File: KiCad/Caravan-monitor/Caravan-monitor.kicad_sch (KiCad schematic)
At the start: 14 parts, among them IC2 STM32L011F4P6TR, J1 Conn_ARM_JTAG_SWD_20, J2 8-28V input, SW1 SW_SPST

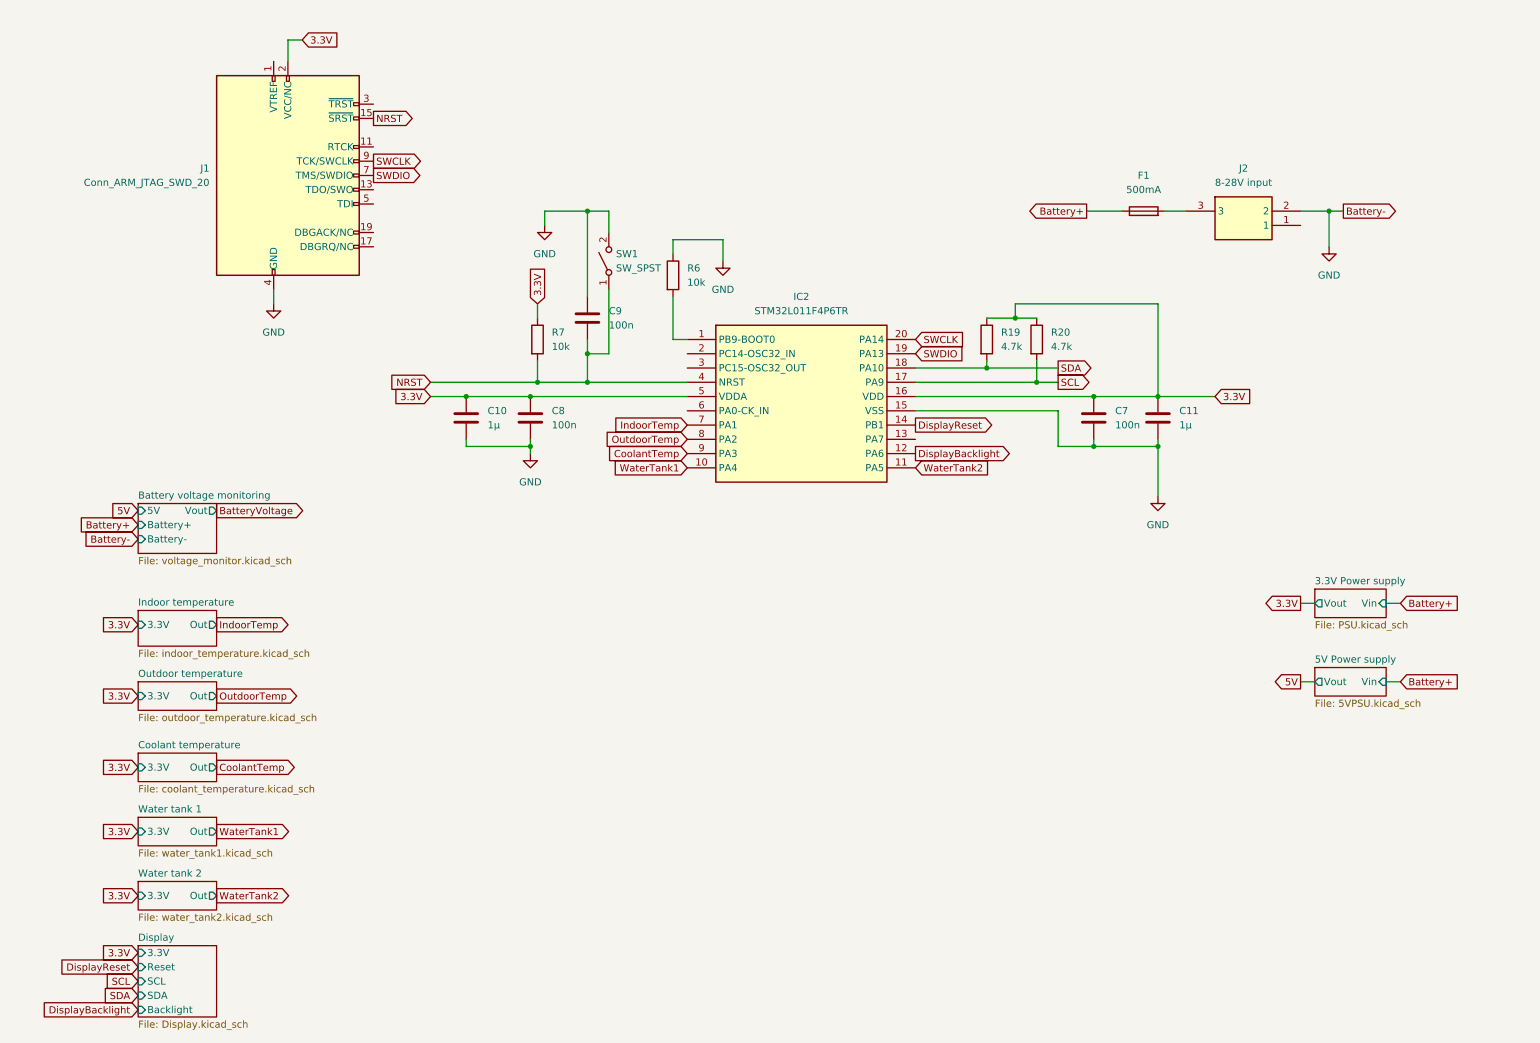
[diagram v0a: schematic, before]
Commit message: Schematics done
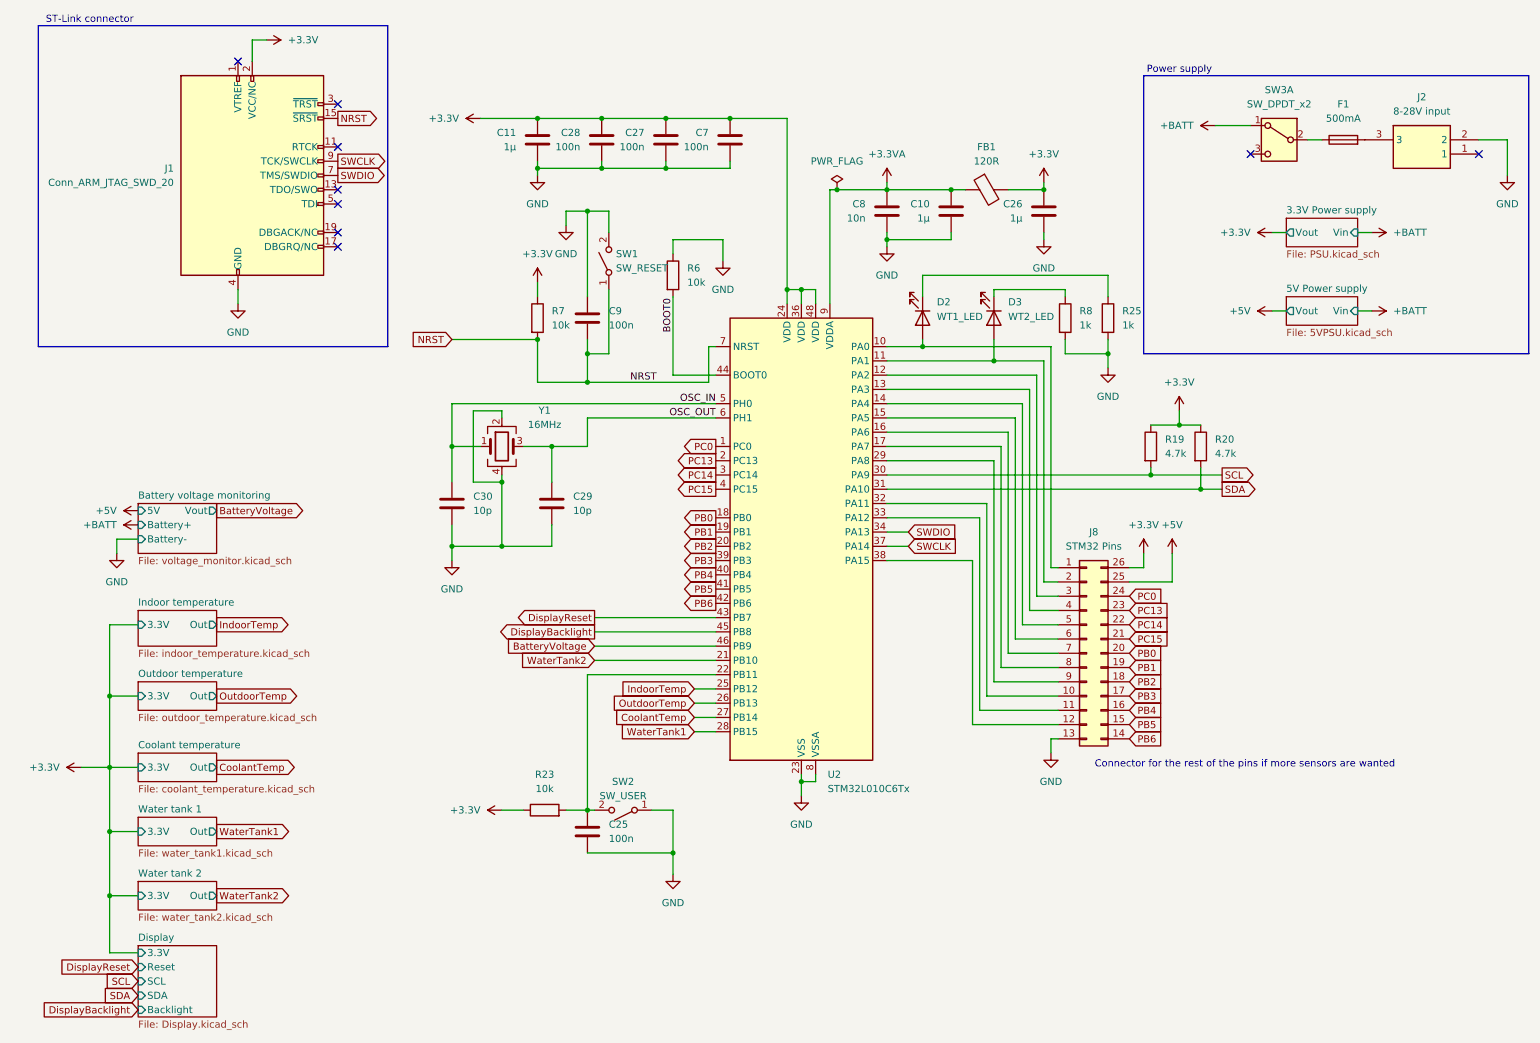
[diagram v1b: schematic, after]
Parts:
- removed IC2: STM32L011F4P6TR, SamacSys_Parts:SOP65P640X120-20N, symbol SamacSys_Parts:STM32L011F4P6TR
- added C25, C27, C28: 100n, Capacitor_SMD:C_0402_1005Metric_Pad0.74x0.62mm_HandSolder, symbol Device:C
- added C26: 1µ, Capacitor_SMD:C_0402_1005Metric_Pad0.74x0.62mm_HandSolder, symbol Device:C
- added C29, C30: 10p, Capacitor_SMD:C_0402_1005Metric_Pad0.74x0.62mm_HandSolder, symbol Device:C
- added D2: WT1_LED, LED_SMD:LED_0402_1005Metric_Pad0.77x0.64mm_HandSolder, symbol Device:LED
- added D3: WT2_LED, LED_SMD:LED_0402_1005Metric_Pad0.77x0.64mm_HandSolder, symbol Device:LED
- added FB1: 120R, Inductor_SMD:L_0402_1005Metric_Pad0.77x0.64mm_HandSolder, symbol Device:FerriteBead
- added J8: STM32 Pins, Connector_PinHeader_2.54mm:PinHeader_2x13_P2.54mm_Horizontal, symbol Connector_Generic:Conn_02x13_Counter_Clockwise
- added R23: 10k, Resistor_SMD:R_0402_1005Metric_Pad0.72x0.64mm_HandSolder, symbol Device:R
- added R25, R8: 1k, Resistor_SMD:R_0402_1005Metric_Pad0.72x0.64mm_HandSolder, symbol Device:R
- added SW2: SW_USER, Button_Switch_SMD:SW_SPST_PTS645, symbol Switch:SW_SPST
- added SW3: SW_DPDT_x2, Button_Switch_THT:SW_E-Switch_EG2219_DPDT_Angled, symbol Switch:SW_DPDT_x2
- added U2: STM32L010C6Tx, Package_QFP:LQFP-48_7x7mm_P0.5mm, symbol MCU_ST_STM32L0:STM32L010C6Tx
- added Y1: 16MHz, symbol Device:Crystal_GND24
- C10, C11, C7, C9: footprint Capacitor_SMD:C_0805_2012Metric_Pad1.18x1.45mm_HandSolder -> Capacitor_SMD:C_0402_1005Metric_Pad0.74x0.62mm_HandSolder
- C8: value 100n -> 10n; footprint Capacitor_SMD:C_0805_2012Metric_Pad1.18x1.45mm_HandSolder -> Capacitor_SMD:C_0402_1005Metric_Pad0.74x0.62mm_HandSolder
- R19, R20, R6, R7: footprint Resistor_SMD:R_0805_2012Metric_Pad1.20x1.40mm_HandSolder -> Resistor_SMD:R_0402_1005Metric_Pad0.72x0.64mm_HandSolder
- SW1: value SW_SPST -> SW_RESET
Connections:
- net BatteryVoltage: now also U2.46 (PB9)
- net CoolantTemp: now also U2.27 (PB14)
- net DisplayBacklight: now also U2.45 (PB8)
- net DisplayReset: now also U2.43 (PB7)
- net GND: now also C25.1, C26.2, C27.2, C28.2, C29.2, C30.2, J8.13 (Pin_13), R25.2, R8.2, SW2.1 (A), U2.23 (VSS), U2.35 (VSS), U2.47 (VSS), U2.8 (VSSA), Y1.2, Y1.4
- net IndoorTemp: now also U2.25 (PB12)
- net NRST: now also U2.7 (NRST)
- net OutdoorTemp: now also U2.26 (PB13)
- net SCL: now also R19.2, U2.30 (PA9); no longer R20.2
- net SDA: now also R20.2, U2.31 (PA10); no longer R19.2
- net SWCLK: now also U2.37 (PA14)
- net SWDIO: now also U2.34 (PA13)
- net WaterTank1: now also U2.28 (PB15)
- net WaterTank2: now also U2.21 (PB10)
- net BOOT0: now reaches R6.2
- net BOOT0: now also U2.44 (BOOT0)
- net 3.3V renamed +3.3V
- net +3.3V: now also C26.1, C27.1, C28.1, FB1.2, J8.26 (Pin_26), R23.1, U2.24 (VDD), U2.36 (VDD), U2.48 (VDD); no longer C10.1, C8.1
- net Battery+: no longer names the net of F1.1
- net Battery+: now also SW3.2 (B)
- new net: D2.2 (A), J8.1 (Pin_1), U2.10 (PA0)
- new net: J8.10 (Pin_10), U2.32 (PA11)
- new net: J8.11 (Pin_11), U2.33 (PA12)
- new net: J8.12 (Pin_12), U2.38 (PA15)
- new net: D3.2 (A), J8.2 (Pin_2), U2.11 (PA1)
- new net: J8.3 (Pin_3), U2.12 (PA2)
- new net: J8.4 (Pin_4), U2.13 (PA3)
- new net: J8.5 (Pin_5), U2.14 (PA4)
- new net: J8.6 (Pin_6), U2.15 (PA5)
- new net: J8.7 (Pin_7), U2.16 (PA6)
- new net: J8.8 (Pin_8), U2.17 (PA7)
- new net: J8.9 (Pin_9), U2.29 (PA8)
- new net: C25.2, R23.2, SW2.2 (B), U2.22 (PB11)
- new net: D3.1 (K), R8.1
- new net: D2.1 (K), R25.1
- new net +3.3VA: C10.1, C8.1, FB1.1, U2.9 (VDDA)
- new net +5V: J8.25 (Pin_25)
- new net +BATT: SW3.1 (A)
- new net OSC_IN: C30.1, U2.5 (PH0), Y1.1
- new net OSC_OUT: C29.1, U2.6 (PH1), Y1.3
- new net PB0: J8.20 (Pin_20), U2.18 (PB0)
- new net PB1: J8.19 (Pin_19), U2.19 (PB1)
- new net PB2: J8.18 (Pin_18), U2.20 (PB2)
- new net PB3: J8.17 (Pin_17), U2.39 (PB3)
- new net PB4: J8.16 (Pin_16), U2.40 (PB4)
- new net PB5: J8.15 (Pin_15), U2.41 (PB5)
- new net PB6: J8.14 (Pin_14), U2.42 (PB6)
- new net PC0: J8.24 (Pin_24), U2.1 (PC0)
- new net PC13: J8.23 (Pin_23), U2.2 (PC13)
- new net PC14: J8.22 (Pin_22), U2.3 (PC14)
- new net PC15: J8.21 (Pin_21), U2.4 (PC15)
- no-connect marks 0 -> 9
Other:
- note added: "Connector for the rest of the pins if more sensors are wanted"
- note added: "Power supply"
- note added: "ST-Link connector"
- moved on the sheet: C10, C11, C7, C8, F1, J1, J2, R19, R20, R7
